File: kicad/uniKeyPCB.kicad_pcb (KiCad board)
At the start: 2 copper layers, 84 x 84 mm, 136 parts, among them J1 Conn_01x03_Socket, J10 Conn_01x02_Socket, J2 Conn_01x03_Socket, J3 Conn_01x02_Socket, J4 Conn_01x02_Socket, J5 Conn_01x03_Socket, J6 Conn_01x03_Socket, J9 Conn_01x02_Socket, SW1 SW_CHOC_HS, SW2 SW_MX_HS

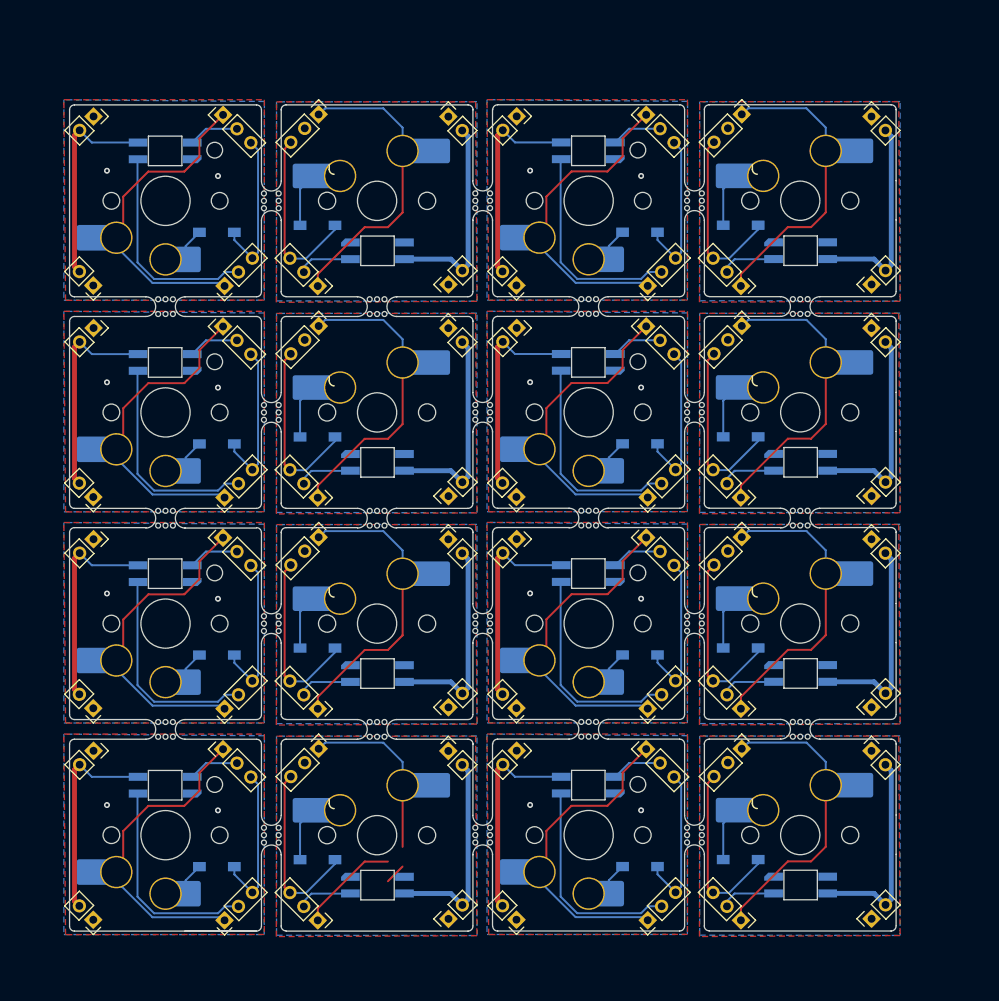
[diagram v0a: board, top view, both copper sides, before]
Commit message: bug fix (#2)
* amended reamnd

* fixed a bug
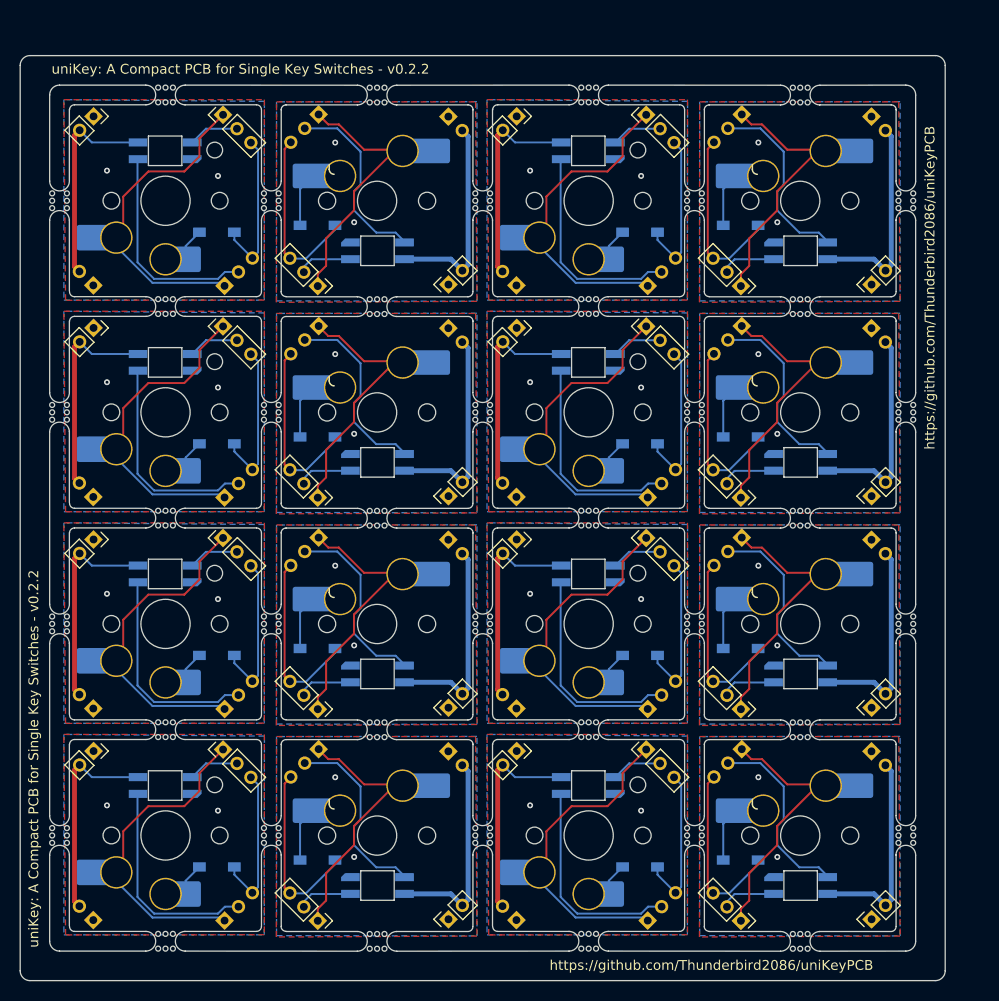
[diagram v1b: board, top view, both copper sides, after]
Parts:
- removed the D1 at (75.5, 130.6)
- removed the D1 at (118.6, 130.6)
- removed the D1 at (75.5, 87.6)
- removed the D1 at (75.5, 109.1)
- removed the D1 at (75.5, 66.1)
- removed the D1 at (118.6, 109.0)
- removed the D2 at (128.8, 129.8)
- removed the D2 at (128.8, 65.4)
- removed the D2 at (85.8, 129.8)
- removed the D2 at (128.8, 108.3)
- removed the D2 at (128.8, 86.9)
- removed the D2 at (85.8, 108.3)
- removed the J1 at (119.2, 118.6)
- removed the J1 at (76.2, 54.2)
- removed the J1 at (76.2, 75.7)
- removed the J1 at (119.2, 97.1)
- removed the J1 at (76.2, 97.1)
- removed the J1 at (76.2, 118.6)
- removed the J10 at (63.0, 136.0)
- removed the J10 at (106.0, 114.5)
- removed the J10 at (63.0, 93.0)
- removed the J10 at (63.0, 114.5)
- removed the J10 at (106.0, 135.9)
- removed the J10 at (63.0, 71.5)
- removed the J2 at (76.3, 71.5)
- removed the J2 at (76.3, 114.5)
- removed the J2 at (119.3, 136.0)
- removed the J2 at (76.3, 136.0)
- removed the J2 at (76.3, 93.0)
- removed the J2 at (119.3, 114.5)
- removed the J3 at (142.1, 71.4)
- removed the J3 at (99.1, 114.4)
- removed the J3 at (142.1, 135.9)
- removed the J3 at (99.1, 135.9)
- removed the J3 at (142.1, 114.4)
- removed the J3 at (142.1, 92.9)
- removed the J4 at (142.1, 97.3)
- removed the J4 at (142.1, 118.8)
- removed the J4 at (142.1, 75.8)
- removed the J4 at (99.1, 118.8)
- removed the J4 at (142.1, 54.3)
- removed the J4 at (99.1, 97.3)
- removed the J5 at (128.8, 114.5)
- removed the J5 at (85.8, 136.0)
- removed the J5 at (85.8, 114.5)
- removed the J5 at (128.8, 136.0)
- removed the J5 at (128.8, 93.0)
- removed the J5 at (128.8, 71.5)
- removed the J6 at (85.9, 118.6)
- removed the J6 at (128.9, 54.1)
- removed the J6 at (128.9, 118.6)
- removed the J6 at (128.9, 75.6)
- removed the J6 at (128.9, 97.1)
- removed the J6 at (85.9, 97.1)
- removed the J9 at (63.0, 118.8)
- removed the J9 at (106.0, 97.3)
- removed the J9 at (63.0, 97.3)
- removed the J9 at (63.0, 75.8)
- removed the J9 at (106.0, 118.8)
- removed the J9 at (63.0, 54.3)
- removed the LED1 at (113.3, 122.3)
- removed the LED1 at (70.3, 100.8)
- removed the LED1 at (70.3, 79.3)
- removed the LED1 at (113.3, 100.8)
- removed the LED1 at (70.3, 57.8)
- removed the LED1 at (70.3, 122.3)
- removed the LED2 at (134.8, 89.5)
- removed the LED2 at (134.8, 110.9)
- removed the LED2 at (91.8, 110.9)
- removed the LED2 at (91.8, 132.4)
- removed the LED2 at (134.8, 68.0)
- removed the LED2 at (134.8, 132.4)
- removed the SW1 at (70.3, 62.9)
- removed the SW1 at (113.3, 127.3)
- removed the SW1 at (113.3, 105.8)
- removed the SW1 at (70.3, 105.9)
- removed the SW1 at (70.3, 127.4)
- removed the SW1 at (70.3, 84.4)
- removed the SW2 at (134.8, 127.3)
- removed the SW2 at (134.8, 105.8)
- removed the SW2 at (134.8, 62.9)
- removed the SW2 at (91.8, 127.4)
- removed the SW2 at (134.8, 84.4)
- removed the SW2 at (91.8, 105.9)
- removed the mouse-bite-2mm-slot at (81.1, 62.9)
- removed the mouse-bite-2mm-slot at (70.3, 95.2)
- removed the mouse-bite-2mm-slot at (102.6, 127.3)
- removed the mouse-bite-2mm-slot at (102.6, 105.8)
- removed the mouse-bite-2mm-slot at (70.3, 73.7)
- removed the mouse-bite-2mm-slot at (124.1, 127.3)
- removed the mouse-bite-2mm-slot at (124.1, 105.8)
- removed the mouse-bite-2mm-slot at (91.8, 116.6)
- removed the mouse-bite-2mm-slot at (134.8, 73.6)
- removed the mouse-bite-2mm-slot at (113.3, 116.6)
- removed the mouse-bite-2mm-slot at (81.1, 127.4)
- removed the mouse-bite-2mm-slot at (81.1, 84.4)
- removed the mouse-bite-2mm-slot at (134.8, 116.6)
- removed the mouse-bite-2mm-slot at (134.8, 95.1)
- removed the mouse-bite-2mm-slot at (81.1, 105.9)
- removed the mouse-bite-2mm-slot at (70.3, 116.6)
- added D1: 1N4148WS, TB2086_SMD:D3_SMD, F.Cu at (75.6, 66.1)
- added D1: 1N4148WS, TB2086_SMD:D3_SMD, F.Cu at (75.6, 109.1)
- added D1: 1N4148WS, TB2086_SMD:D3_SMD, F.Cu at (75.6, 87.6)
- added D1: 1N4148WS, TB2086_SMD:D3_SMD, F.Cu at (75.6, 130.6)
- added D1: 1N4148WS, TB2086_SMD:D3_SMD, F.Cu at (118.6, 109.1)
- added D1: 1N4148WS, TB2086_SMD:D3_SMD, F.Cu at (118.6, 130.6)
- added D2: 1N4148WS, TB2086_SMD:D3_SMD, F.Cu at (85.8, 108.4)
- added D2: 1N4148WS, TB2086_SMD:D3_SMD, F.Cu at (128.8, 65.4)
- added D2: 1N4148WS, TB2086_SMD:D3_SMD, F.Cu at (128.8, 86.9)
- added D2: 1N4148WS, TB2086_SMD:D3_SMD, F.Cu at (128.8, 108.4)
- added D2: 1N4148WS, TB2086_SMD:D3_SMD, F.Cu at (85.8, 129.9)
- added D2: 1N4148WS, TB2086_SMD:D3_SMD, F.Cu at (128.8, 129.9)
- added J1: Conn_01x03_Socket, Connector_PinHeader_2.00mm:PinHeader_1x03_P2.00mm_Vertical, F.Cu at (119.2, 118.7)
- added J1: Conn_01x03_Socket, Connector_PinHeader_2.00mm:PinHeader_1x03_P2.00mm_Vertical, F.Cu at (119.2, 97.2)
- added J1: Conn_01x03_Socket, Connector_PinHeader_2.00mm:PinHeader_1x03_P2.00mm_Vertical, F.Cu at (76.2, 54.2)
- added J1: Conn_01x03_Socket, Connector_PinHeader_2.00mm:PinHeader_1x03_P2.00mm_Vertical, F.Cu at (76.2, 118.7)
- added J1: Conn_01x03_Socket, Connector_PinHeader_2.00mm:PinHeader_1x03_P2.00mm_Vertical, F.Cu at (76.2, 75.7)
- added J1: Conn_01x03_Socket, Connector_PinHeader_2.00mm:PinHeader_1x03_P2.00mm_Vertical, F.Cu at (76.2, 97.2)
- added J10: Conn_01x02_Socket, Connector_PinSocket_2.00mm:PinSocket_1x02_P2.00mm_Vertical, B.Cu at (106.0, 114.5)
- added J10: Conn_01x02_Socket, Connector_PinSocket_2.00mm:PinSocket_1x02_P2.00mm_Vertical, B.Cu at (63.0, 93.0)
- added J10: Conn_01x02_Socket, Connector_PinSocket_2.00mm:PinSocket_1x02_P2.00mm_Vertical, B.Cu at (63.0, 136.0)
- added J10: Conn_01x02_Socket, Connector_PinSocket_2.00mm:PinSocket_1x02_P2.00mm_Vertical, B.Cu at (106.0, 136.0)
- added J10: Conn_01x02_Socket, Connector_PinSocket_2.00mm:PinSocket_1x02_P2.00mm_Vertical, B.Cu at (63.0, 71.5)
- added J10: Conn_01x02_Socket, Connector_PinSocket_2.00mm:PinSocket_1x02_P2.00mm_Vertical, B.Cu at (63.0, 114.5)
- added J2: Conn_01x03_Socket, Connector_PinHeader_2.00mm:PinHeader_1x03_P2.00mm_Vertical, B.Cu at (76.3, 136.0)
- added J2: Conn_01x03_Socket, Connector_PinHeader_2.00mm:PinHeader_1x03_P2.00mm_Vertical, B.Cu at (119.3, 114.5)
- added J2: Conn_01x03_Socket, Connector_PinHeader_2.00mm:PinHeader_1x03_P2.00mm_Vertical, B.Cu at (119.3, 136.0)
- added J2: Conn_01x03_Socket, Connector_PinHeader_2.00mm:PinHeader_1x03_P2.00mm_Vertical, B.Cu at (76.3, 114.5)
- added J2: Conn_01x03_Socket, Connector_PinHeader_2.00mm:PinHeader_1x03_P2.00mm_Vertical, B.Cu at (76.3, 93.0)
- added J2: Conn_01x03_Socket, Connector_PinHeader_2.00mm:PinHeader_1x03_P2.00mm_Vertical, B.Cu at (76.3, 71.5)
- added J3: Conn_01x02_Socket, Connector_PinSocket_2.00mm:PinSocket_1x02_P2.00mm_Vertical, F.Cu at (142.1, 92.9)
- added J3: Conn_01x02_Socket, Connector_PinSocket_2.00mm:PinSocket_1x02_P2.00mm_Vertical, F.Cu at (99.1, 135.9)
- added J3: Conn_01x02_Socket, Connector_PinSocket_2.00mm:PinSocket_1x02_P2.00mm_Vertical, F.Cu at (99.1, 114.4)
- added J3: Conn_01x02_Socket, Connector_PinSocket_2.00mm:PinSocket_1x02_P2.00mm_Vertical, F.Cu at (142.1, 114.4)
- added J3: Conn_01x02_Socket, Connector_PinSocket_2.00mm:PinSocket_1x02_P2.00mm_Vertical, F.Cu at (142.1, 71.4)
- added J3: Conn_01x02_Socket, Connector_PinSocket_2.00mm:PinSocket_1x02_P2.00mm_Vertical, F.Cu at (142.1, 135.9)
- added J4: Conn_01x02_Socket, Connector_PinSocket_2.00mm:PinSocket_1x02_P2.00mm_Vertical, B.Cu at (99.1, 97.3)
- added J4: Conn_01x02_Socket, Connector_PinSocket_2.00mm:PinSocket_1x02_P2.00mm_Vertical, B.Cu at (142.1, 75.8)
- added J4: Conn_01x02_Socket, Connector_PinSocket_2.00mm:PinSocket_1x02_P2.00mm_Vertical, B.Cu at (142.1, 97.3)
- added J4: Conn_01x02_Socket, Connector_PinSocket_2.00mm:PinSocket_1x02_P2.00mm_Vertical, B.Cu at (99.1, 118.8)
- added J4: Conn_01x02_Socket, Connector_PinSocket_2.00mm:PinSocket_1x02_P2.00mm_Vertical, B.Cu at (142.1, 54.3)
- added J4: Conn_01x02_Socket, Connector_PinSocket_2.00mm:PinSocket_1x02_P2.00mm_Vertical, B.Cu at (142.1, 118.8)
- added J5: Conn_01x03_Socket, Connector_PinHeader_2.00mm:PinHeader_1x03_P2.00mm_Vertical, F.Cu at (128.8, 114.6)
- added J5: Conn_01x03_Socket, Connector_PinHeader_2.00mm:PinHeader_1x03_P2.00mm_Vertical, F.Cu at (128.8, 136.1)
- added J5: Conn_01x03_Socket, Connector_PinHeader_2.00mm:PinHeader_1x03_P2.00mm_Vertical, F.Cu at (85.8, 114.6)
- added J5: Conn_01x03_Socket, Connector_PinHeader_2.00mm:PinHeader_1x03_P2.00mm_Vertical, F.Cu at (128.8, 93.1)
- added J5: Conn_01x03_Socket, Connector_PinHeader_2.00mm:PinHeader_1x03_P2.00mm_Vertical, F.Cu at (128.8, 71.6)
- added J5: Conn_01x03_Socket, Connector_PinHeader_2.00mm:PinHeader_1x03_P2.00mm_Vertical, F.Cu at (85.8, 136.1)
- added J6: Conn_01x03_Socket, Connector_PinHeader_2.00mm:PinHeader_1x03_P2.00mm_Vertical, B.Cu at (128.9, 97.1)
- added J6: Conn_01x03_Socket, Connector_PinHeader_2.00mm:PinHeader_1x03_P2.00mm_Vertical, B.Cu at (128.9, 75.6)
- added J6: Conn_01x03_Socket, Connector_PinHeader_2.00mm:PinHeader_1x03_P2.00mm_Vertical, B.Cu at (128.9, 54.1)
- added J6: Conn_01x03_Socket, Connector_PinHeader_2.00mm:PinHeader_1x03_P2.00mm_Vertical, B.Cu at (128.9, 118.6)
- added J6: Conn_01x03_Socket, Connector_PinHeader_2.00mm:PinHeader_1x03_P2.00mm_Vertical, B.Cu at (85.9, 118.6)
- added J6: Conn_01x03_Socket, Connector_PinHeader_2.00mm:PinHeader_1x03_P2.00mm_Vertical, B.Cu at (85.9, 97.1)
- added J9: Conn_01x02_Socket, Connector_PinSocket_2.00mm:PinSocket_1x02_P2.00mm_Vertical, F.Cu at (63.0, 75.8)
- added J9: Conn_01x02_Socket, Connector_PinSocket_2.00mm:PinSocket_1x02_P2.00mm_Vertical, F.Cu at (63.0, 97.3)
- added J9: Conn_01x02_Socket, Connector_PinSocket_2.00mm:PinSocket_1x02_P2.00mm_Vertical, F.Cu at (106.0, 118.8)
- added J9: Conn_01x02_Socket, Connector_PinSocket_2.00mm:PinSocket_1x02_P2.00mm_Vertical, F.Cu at (106.0, 97.3)
- added J9: Conn_01x02_Socket, Connector_PinSocket_2.00mm:PinSocket_1x02_P2.00mm_Vertical, F.Cu at (63.0, 118.8)
- added J9: Conn_01x02_Socket, Connector_PinSocket_2.00mm:PinSocket_1x02_P2.00mm_Vertical, F.Cu at (63.0, 54.3)
- added LED1: SK6812MINI-E, TB2086_LED:LED_SW_SK6812-E-rot, F.Cu at (113.3, 100.8)
- added LED1: SK6812MINI-E, TB2086_LED:LED_SW_SK6812-E-rot, F.Cu at (70.3, 100.8)
- added LED1: SK6812MINI-E, TB2086_LED:LED_SW_SK6812-E-rot, F.Cu at (70.3, 79.3)
- added LED1: SK6812MINI-E, TB2086_LED:LED_SW_SK6812-E-rot, F.Cu at (113.3, 122.3)
- added LED1: SK6812MINI-E, TB2086_LED:LED_SW_SK6812-E-rot, F.Cu at (70.3, 122.3)
- added LED1: SK6812MINI-E, TB2086_LED:LED_SW_SK6812-E-rot, F.Cu at (70.3, 57.8)
- added LED2: SK6812MINI-E, TB2086_LED:LED_SW_SK6812-E-rot, F.Cu at (134.8, 89.5)
- added LED2: SK6812MINI-E, TB2086_LED:LED_SW_SK6812-E-rot, F.Cu at (134.8, 68.0)
- added LED2: SK6812MINI-E, TB2086_LED:LED_SW_SK6812-E-rot, F.Cu at (134.8, 111.0)
- added LED2: SK6812MINI-E, TB2086_LED:LED_SW_SK6812-E-rot, F.Cu at (134.8, 132.5)
- added LED2: SK6812MINI-E, TB2086_LED:LED_SW_SK6812-E-rot, F.Cu at (91.8, 111.0)
- added LED2: SK6812MINI-E, TB2086_LED:LED_SW_SK6812-E-rot, F.Cu at (91.8, 132.5)
- added SW1: SW_CHOC_HS, TB2086_KEYSWITCH:SW_choc_v1_v2_HS_1u, F.Cu at (113.3, 105.9)
- added SW1: SW_CHOC_HS, TB2086_KEYSWITCH:SW_choc_v1_v2_HS_1u, F.Cu at (70.3, 84.4)
- added SW1: SW_CHOC_HS, TB2086_KEYSWITCH:SW_choc_v1_v2_HS_1u, F.Cu at (70.3, 62.9)
- added SW1: SW_CHOC_HS, TB2086_KEYSWITCH:SW_choc_v1_v2_HS_1u, F.Cu at (70.3, 105.9)
- added SW1: SW_CHOC_HS, TB2086_KEYSWITCH:SW_choc_v1_v2_HS_1u, F.Cu at (70.3, 127.4)
- added SW1: SW_CHOC_HS, TB2086_KEYSWITCH:SW_choc_v1_v2_HS_1u, F.Cu at (113.3, 127.4)
- added SW2: SW_MX_HS, TB2086_KEYSWITCH:SW_MX_HS_1u, F.Cu at (91.8, 127.4)
- added SW2: SW_MX_HS, TB2086_KEYSWITCH:SW_MX_HS_1u, F.Cu at (134.8, 62.9)
- added SW2: SW_MX_HS, TB2086_KEYSWITCH:SW_MX_HS_1u, F.Cu at (134.8, 105.9)
- added SW2: SW_MX_HS, TB2086_KEYSWITCH:SW_MX_HS_1u, F.Cu at (134.8, 127.4)
- added SW2: SW_MX_HS, TB2086_KEYSWITCH:SW_MX_HS_1u, F.Cu at (134.8, 84.4)
- added SW2: SW_MX_HS, TB2086_KEYSWITCH:SW_MX_HS_1u, F.Cu at (91.8, 105.9)
- added mouse-bite-2mm-slot: VAL**, Mouse_Bite:mouse-bite-2mm-slot, F.Cu at (81.1, 84.4)
- added mouse-bite-2mm-slot: VAL**, Mouse_Bite:mouse-bite-2mm-slot, F.Cu at (113.3, 116.6)
- added mouse-bite-2mm-slot: VAL**, Mouse_Bite:mouse-bite-2mm-slot, F.Cu at (91.8, 116.7)
- added mouse-bite-2mm-slot: VAL**, Mouse_Bite:mouse-bite-2mm-slot, F.Cu at (59.6, 127.4)
- added mouse-bite-2mm-slot: VAL**, Mouse_Bite:mouse-bite-2mm-slot, F.Cu at (102.6, 105.9)
- added mouse-bite-2mm-slot: VAL**, Mouse_Bite:mouse-bite-2mm-slot, F.Cu at (145.6, 84.4)
- added mouse-bite-2mm-slot: VAL**, Mouse_Bite:mouse-bite-2mm-slot, F.Cu at (145.6, 62.9)
- added mouse-bite-2mm-slot: VAL**, Mouse_Bite:mouse-bite-2mm-slot, F.Cu at (124.1, 127.4)
- added mouse-bite-2mm-slot: VAL**, Mouse_Bite:mouse-bite-2mm-slot, F.Cu at (145.6, 127.4)
- added mouse-bite-2mm-slot: VAL**, Mouse_Bite:mouse-bite-2mm-slot, F.Cu at (81.1, 127.4)
- added mouse-bite-2mm-slot: VAL**, Mouse_Bite:mouse-bite-2mm-slot, F.Cu at (113.3, 138.1)
- added mouse-bite-2mm-slot: VAL**, Mouse_Bite:mouse-bite-2mm-slot, F.Cu at (70.3, 73.6)
- added mouse-bite-2mm-slot: VAL**, Mouse_Bite:mouse-bite-2mm-slot, F.Cu at (134.8, 116.7)
- added mouse-bite-2mm-slot: VAL**, Mouse_Bite:mouse-bite-2mm-slot, F.Cu at (81.1, 62.9)
- added mouse-bite-2mm-slot: VAL**, Mouse_Bite:mouse-bite-2mm-slot, F.Cu at (70.3, 52.1)
- added mouse-bite-2mm-slot: VAL**, Mouse_Bite:mouse-bite-2mm-slot, F.Cu at (134.8, 138.2)
- added mouse-bite-2mm-slot: VAL**, Mouse_Bite:mouse-bite-2mm-slot, F.Cu at (113.3, 52.1)
- added mouse-bite-2mm-slot: VAL**, Mouse_Bite:mouse-bite-2mm-slot, F.Cu at (134.8, 73.7)
- added mouse-bite-2mm-slot: VAL**, Mouse_Bite:mouse-bite-2mm-slot, F.Cu at (70.3, 138.1)
- added mouse-bite-2mm-slot: VAL**, Mouse_Bite:mouse-bite-2mm-slot, F.Cu at (59.6, 105.9)
- added mouse-bite-2mm-slot: VAL**, Mouse_Bite:mouse-bite-2mm-slot, F.Cu at (59.6, 84.4)
- added mouse-bite-2mm-slot: VAL**, Mouse_Bite:mouse-bite-2mm-slot, F.Cu at (91.8, 138.2)
- added mouse-bite-2mm-slot: VAL**, Mouse_Bite:mouse-bite-2mm-slot, F.Cu at (70.3, 116.6)
- added mouse-bite-2mm-slot: VAL**, Mouse_Bite:mouse-bite-2mm-slot, F.Cu at (145.6, 105.9)
- added mouse-bite-2mm-slot: VAL**, Mouse_Bite:mouse-bite-2mm-slot, F.Cu at (59.6, 62.9)
- added mouse-bite-2mm-slot: VAL**, Mouse_Bite:mouse-bite-2mm-slot, F.Cu at (134.8, 95.2)
- added mouse-bite-2mm-slot: VAL**, Mouse_Bite:mouse-bite-2mm-slot, F.Cu at (134.8, 52.1)
- added mouse-bite-2mm-slot: VAL**, Mouse_Bite:mouse-bite-2mm-slot, F.Cu at (124.1, 105.9)
- added mouse-bite-2mm-slot: VAL**, Mouse_Bite:mouse-bite-2mm-slot, F.Cu at (102.6, 127.4)
- added mouse-bite-2mm-slot: VAL**, Mouse_Bite:mouse-bite-2mm-slot, F.Cu at (70.3, 95.1)
- added mouse-bite-2mm-slot: VAL**, Mouse_Bite:mouse-bite-2mm-slot, F.Cu at (81.1, 105.9)
- added mouse-bite-2mm-slot: VAL**, Mouse_Bite:mouse-bite-2mm-slot, F.Cu at (91.8, 52.1)
- J10 (x2), J2 (x2), J4 (x2), J6 (x2): moved to B.Cu
- turned J10 to 45 degrees (x2)
- turned J2 to -45 degrees (x2)
- turned J4 to -135 degrees (x2)
- turned J6 to 135 degrees (x2)
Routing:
- net LED1_out: track 0.00 -> 155.5 mm
- net col1: track 243.6 -> 223.0 mm
- net GND: track 2.11 -> 0.00 mm, vias 16 -> 32
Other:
- board size 84 x 84 mm -> 94 x 94 mm
- board text added: "<- VCC ->"
- board text added: "<- row ->"
- board text added: "Whether you're a experienced keyboard builder or a beginner, uniKey provides a convenient solution for creating"
- board text added: "https://github.com/Thunderbird2086/uniKeyPCB"
- board text added: "uniKey: A Compact PCB for Single Key Switches - v0.2.2"
- board text added: "unique and personalized keyboards. Happy building!"
- board text added: "v0.2.2"
- board text removed: "led in"
- board text removed: "row"
